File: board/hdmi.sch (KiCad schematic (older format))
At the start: 2 parts

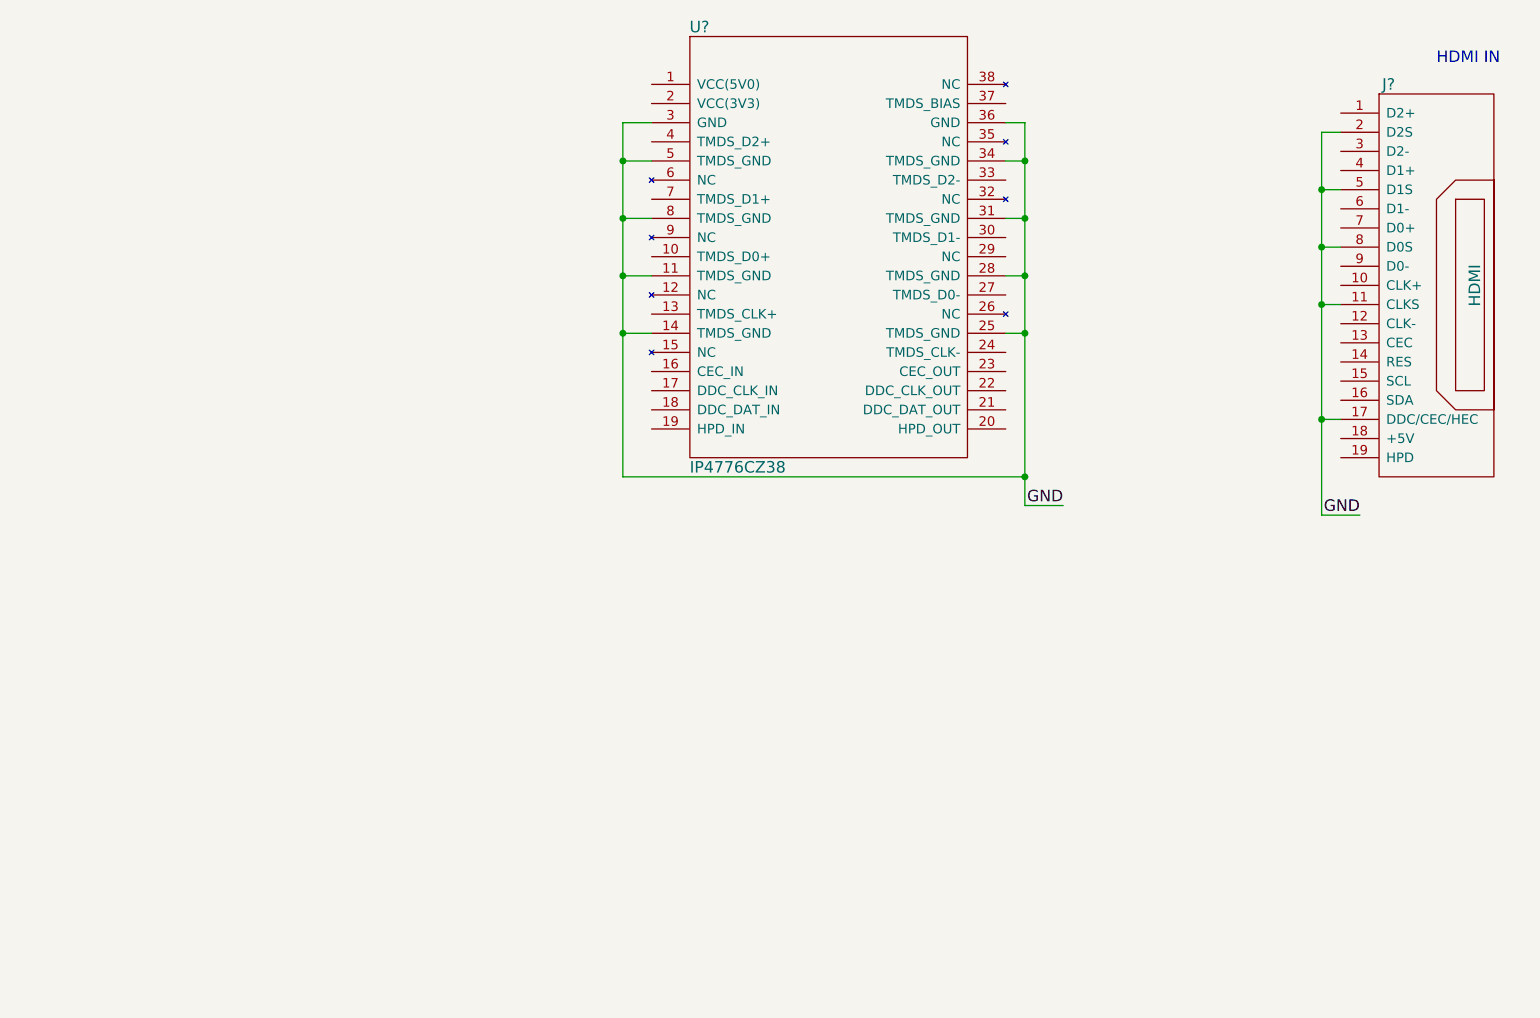
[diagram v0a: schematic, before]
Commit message: Issue #336
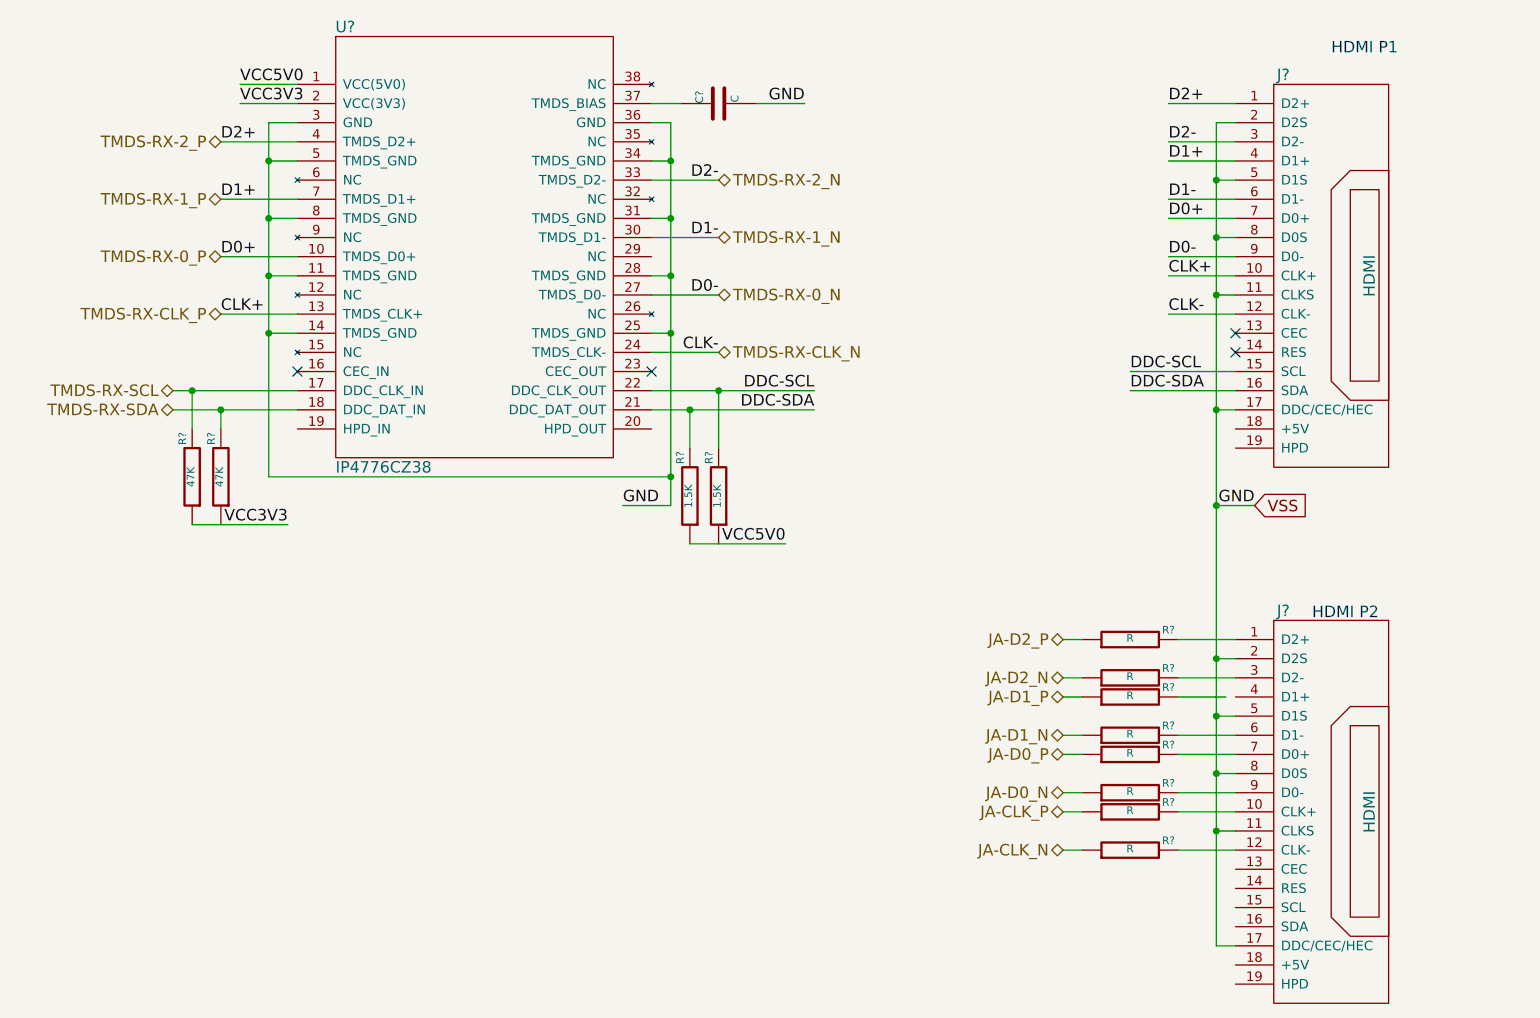
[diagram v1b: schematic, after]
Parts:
- added C?: C, ~, symbol C
- added J?: HDMI, ~, symbol HDMI
- added R? (x8): R, ~, symbol R
- added R? (x2): 1.5K, ~, symbol R
- added R? (x2): 47K, ~, symbol R
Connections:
- net TMDS-RX-2_P: now reaches J?.1 (D2+)
- net TMDS-RX-2_P: now also U?.4 (TMDS_D2+)
- net TMDS-RX-CLK_P: now reaches J?.10 (CLK+)
- net TMDS-RX-CLK_P: now also U?.13 (TMDS_CLK+)
- net TMDS-RX-CLK_N: now reaches J?.12 (CLK-)
- net TMDS-RX-CLK_N: now also U?.24 (TMDS_CLK-)
- net DDC-SCL: now reaches J?.15 (SCL)
- net DDC-SCL: now also U?.22 (DDC_CLK_OUT), R?.2
- net DDC-SDA: now reaches J?.16 (SDA)
- net DDC-SDA: now also U?.21 (DDC_DAT_OUT), R?.2
- net TMDS-RX-2_N: now reaches J?.3 (D2-)
- net TMDS-RX-2_N: now also U?.33 (TMDS_D2-)
- net TMDS-RX-1_P: now reaches J?.4 (D1+)
- net TMDS-RX-1_P: now also U?.7 (TMDS_D1+)
- net TMDS-RX-1_N: now reaches J?.6 (D1-)
- net TMDS-RX-1_N: now also U?.30 (TMDS_D1-)
- net TMDS-RX-0_P: now reaches J?.7 (D0+)
- net TMDS-RX-0_P: now also U?.10 (TMDS_D0+)
- net TMDS-RX-0_N: now reaches J?.9 (D0-)
- net TMDS-RX-0_N: now also U?.27 (TMDS_D0-)
- net VCC5V0: now reaches U?.1 (VCC(5V0))
- net VCC5V0: now also R?.1
- net TMDS-RX-SCL: now reaches U?.17 (DDC_CLK_IN)
- net TMDS-RX-SCL: now also R?.2
- net TMDS-RX-SDA: now reaches U?.18 (DDC_DAT_IN)
- net TMDS-RX-SDA: now also R?.2
- net VCC3V3: now reaches U?.2 (VCC(3V3))
- net VCC3V3: now also R?.1
- net at U?.37 (TMDS_BIAS): now also C?.1
- net GND renamed VSS
- net VSS: now also C?.2, J?.11 (CLKS), J?.17 (DDC/CEC/HEC), J?.2 (D2S), J?.5 (D1S), J?.8 (D0S)
- new net: J?.1 (D2+), R?.2
- new net: J?.10 (CLK+), R?.2
- new net: J?.12 (CLK-), R?.2
- new net: J?.3 (D2-), R?.2
- new net: J?.6 (D1-), R?.2
- new net: J?.7 (D0+), R?.2
- new net: J?.9 (D0-), R?.2
- new net JA-CLK_N: R?.1
- new net JA-CLK_P: R?.1
- new net JA-D0_N: R?.1
- new net JA-D0_P: R?.1
- new net JA-D1_N: R?.1
- new net JA-D1_P: R?.1
- new net JA-D2_N: R?.1
- new net JA-D2_P: R?.1
- no-connect marks 0 -> 4
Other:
- note added: "HDMI P1"
- note added: "HDMI P2"
- note removed: "HDMI IN"
- moved on the sheet: J?, U?
